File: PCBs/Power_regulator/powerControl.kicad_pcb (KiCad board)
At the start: 2 copper layers, 37.8 x 50 mm, 33 parts, among them J1 Conn_01x03_Female, J10 Conn_01x06_Male, J11 Conn_01x04_Male, J2 Conn_01x06_Female, J3 Conn_01x04_Male, J4 Conn_01x01_Male, J5 Conn_01x01_Male, J6 Conn_01x01_Male, J7 Conn_01x01_Male, J8 Conn_01x03_Female, J9 Conn_01x04_Female, Q1 PMOS, Q2 NMOS, Q3 Q_NMOS_GSD, Q4 Q_PMOS_GSD, Q5 Q_NMOS_GSD, U1 MAX9938

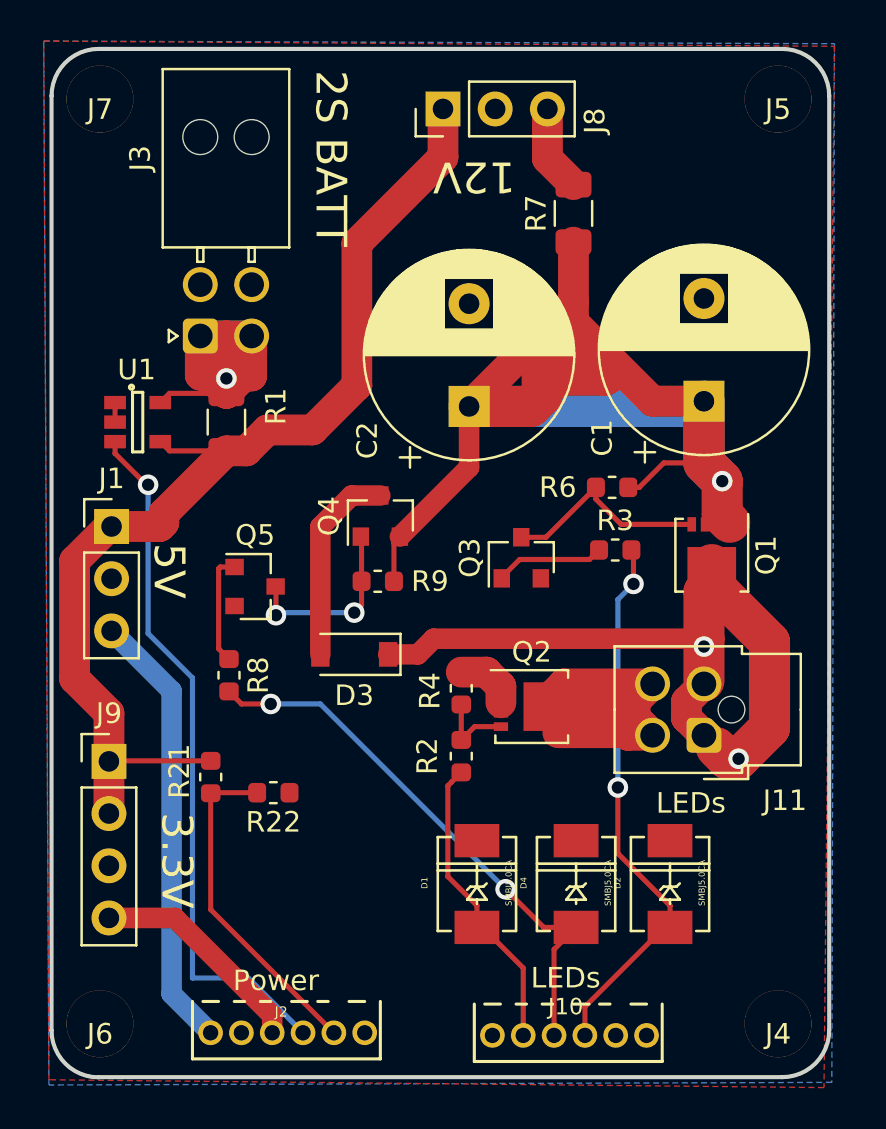
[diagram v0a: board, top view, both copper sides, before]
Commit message: Update for revision05a
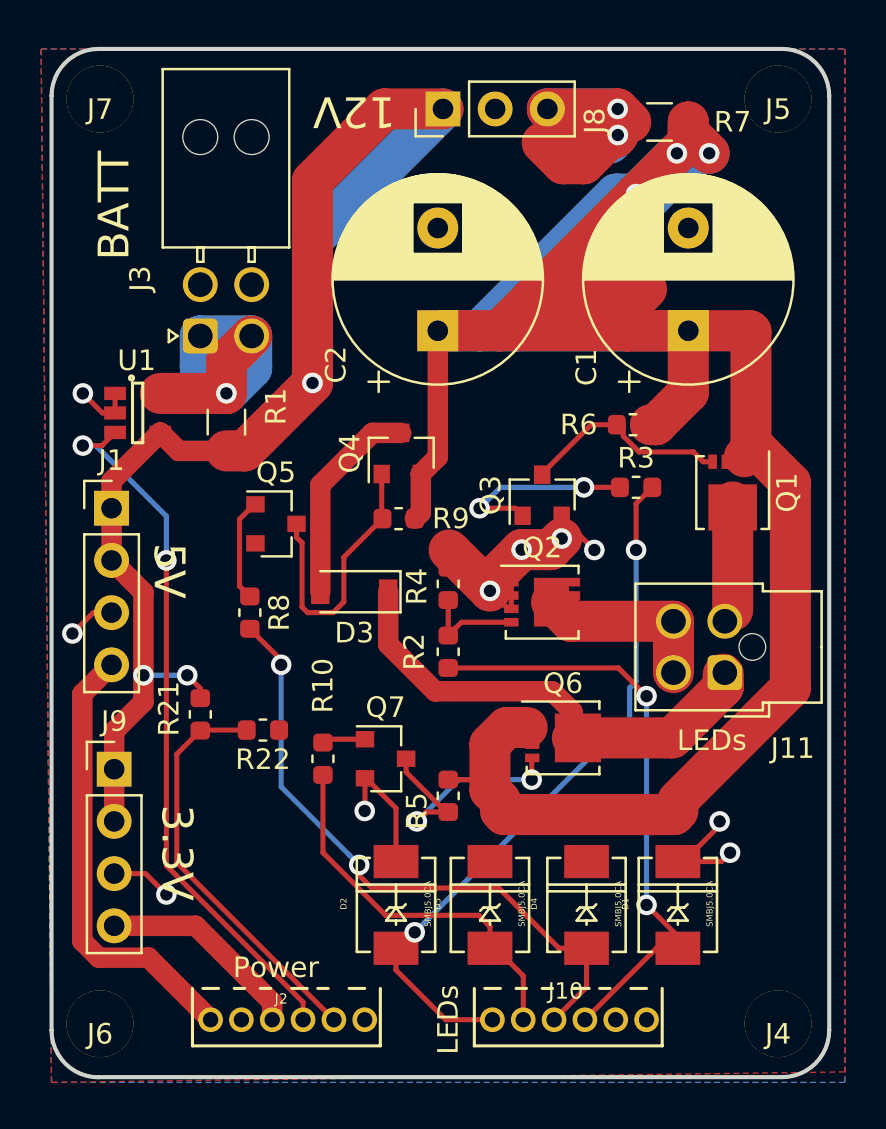
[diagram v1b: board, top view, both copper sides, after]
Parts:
- added D5: SMBJ5.0CA, myLib:DO-214AA, F.Cu at (94.0, 77.2)
- added Q6: PMOS, Package_SON:Diodes_PowerDI3333-8, F.Cu at (97.5, 69.1)
- added Q7: Q_NMOS_GSD, Package_TO_SOT_SMD:SOT-23, F.Cu at (88.9, 70.1)
- added R10: 400R, Resistor_SMD:R_0603_1608Metric, F.Cu at (85.9, 70.1)
- added R5: 10k, Resistor_SMD:R_0603_1608Metric, F.Cu at (91.9, 71.9)
- J1: value Conn_01x03_Female -> Conn_01x04_Female; footprint Connector_PinHeader_2.54mm:PinHeader_1x03_P2.54mm_Vertical -> Connector_PinHeader_2.54mm:PinHeader_1x04_P2.54mm_Vertical
- moved D2 13.4 mm to (89.4, 77.2)
- moved D1 9.83 mm to (103.1, 77.2)
- moved R7 6.11 mm to (102.2, 39.1), turned to 180 degrees
- moved R2 5.12 mm to (91.9, 64.9)
- moved R4 5.12 mm to (91.9, 61.6)
- moved Q2 5.11 mm to (96.5, 62.5)
- moved C2 3.99 mm to (91.4, 49.3)
- moved C1 3.51 mm to (103.6, 49.3)
- moved R8 3.21 mm to (82.3, 63.0)
- moved Q4 3.21 mm to (89.7, 55.2)
- moved Q5 3.21 mm to (83.6, 58.7)
- moved R3 3.21 mm to (101.1, 56.9)
- moved J11 3.21 mm to (105.4, 65.9)
- moved Q1 3.21 mm to (105.8, 57.1)
- moved Q3 3.21 mm to (96.5, 57.3)
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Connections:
- D1 pad 1: LED_EN -> Flash
- D2 pad 1: Flash -> LED_EN2
- D3 pad 1: LED+ -> LED1+
- J1 pad 2: GND -> /Vbatt_out
- J1 pad 3: /5V -> GND
- J10 pad 5: LED_EN -> LED_EN1
- J10 pad 6: LED_Sense -> LED_EN2
- J11 pad 1: LED+ -> LED1+
- J11 pad 2: LED+ -> LED2+
- Q1 pad 5: LED+ -> LED2+
- R2 pad 2: LED_EN -> Flash
- R3 pad 2: Flash -> LED_EN2
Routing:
- net V_LED: track 65.9 -> 140.1 mm, vias 1 -> 3
- net LED+: track 40.3 -> 0.00 mm, vias 2 -> 0
- net LED_EN2: track 0.00 -> 34.4 mm, vias 0 -> 2
- net GND: track 3.96 -> 35.7 mm, vias 0 -> 10
- net LED1+: track 0.00 -> 23.2 mm
- net LED_EN1: track 0.00 -> 18.8 mm
- net /12V: track 4.21 -> 20.7 mm, vias 0 -> 2
- net LED_EN: track 14.8 -> 0.00 mm
- net /Vbatt_out: track 54.1 -> 67.4 mm, vias 0 -> 3
- net Net-(Q6-Pad4): track 0.00 -> 12.7 mm, vias 0 -> 2
- net LED-: track 19.8 -> 8.82 mm
- net /Vbatt_in: track 23.4 -> 15.6 mm
- net LED2+: track 0.00 -> 5.28 mm
- net Net-(Q4-Pad1): track 9.13 -> 13.5 mm, vias 2 -> 0
- net Net-(Q3-Pad1): track 5.34 -> 9.50 mm, vias 0 -> 2
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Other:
- board text added: "BATT"
- board text added: "March 2020"
- board text added: "Power Controller rev04a"
- board text removed: "2S BATT"
- board text removed: "June 25, 2019"
- board text removed: "Power Controller rev03a"

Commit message: Update for BES publication
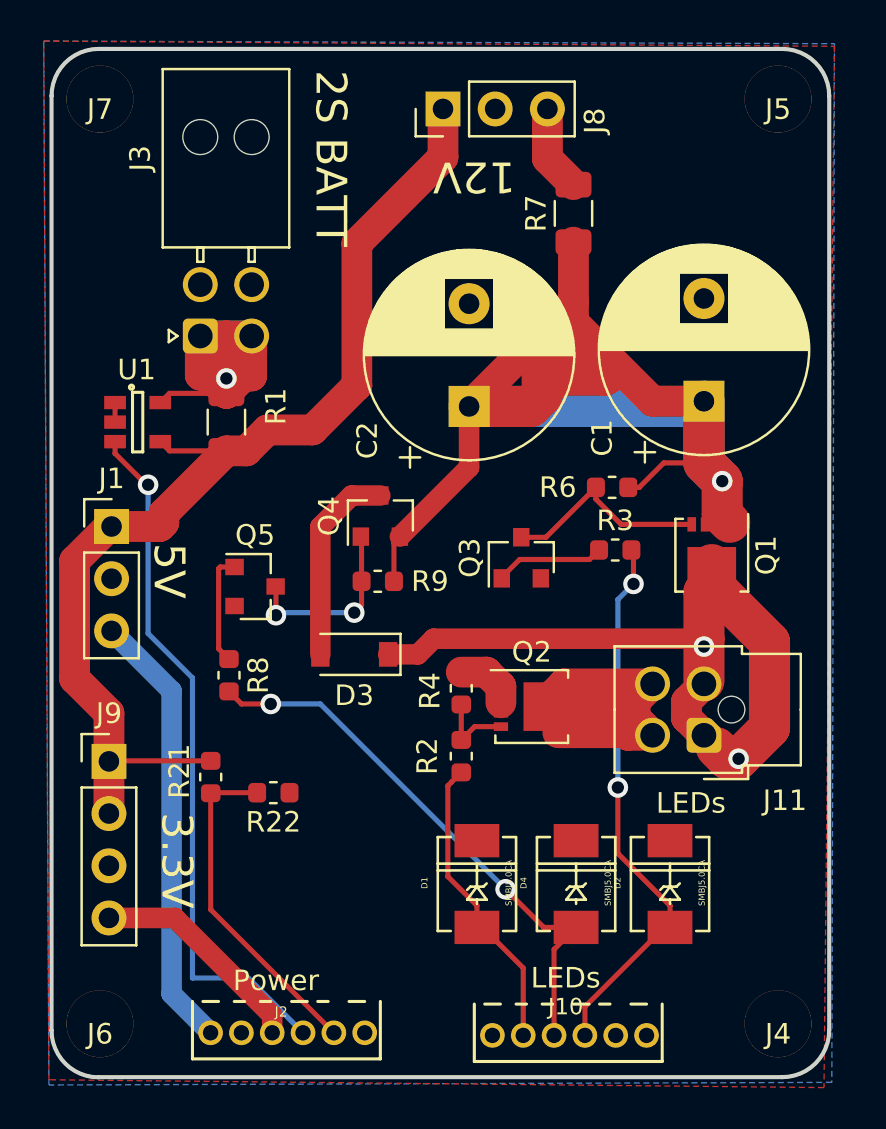
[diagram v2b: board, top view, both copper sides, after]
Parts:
- removed D5: SMBJ5.0CA, myLib:DO-214AA
- removed Q6: PMOS, Package_SON:Diodes_PowerDI3333-8
- removed Q7: Q_NMOS_GSD, Package_TO_SOT_SMD:SOT-23
- removed R10: 400R, Resistor_SMD:R_0603_1608Metric
- removed R5: 10k, Resistor_SMD:R_0603_1608Metric
- J1: value Conn_01x04_Female -> Conn_01x03_Female; footprint Connector_PinHeader_2.54mm:PinHeader_1x04_P2.54mm_Vertical -> Connector_PinHeader_2.54mm:PinHeader_1x03_P2.54mm_Vertical
- moved D2 13.4 mm to (102.7, 76.2)
- moved D1 9.83 mm to (93.3, 76.2)
- moved R7 6.11 mm to (98.0, 43.6), turned to 90 degrees
- moved R2 5.12 mm to (92.6, 70.0)
- moved R4 5.12 mm to (92.6, 66.7)
- moved Q2 5.11 mm to (96.0, 67.6)
- moved C2 3.99 mm to (93.0, 53.0)
- moved C1 3.51 mm to (104.4, 52.7)
- moved R8 3.21 mm to (81.3, 66.0)
- moved Q4 3.21 mm to (88.6, 58.3)
- moved Q5 3.21 mm to (82.5, 61.7)
- moved R3 3.21 mm to (100.1, 59.9)
- moved J11 3.21 mm to (104.4, 69.0)
- moved Q1 3.21 mm to (104.8, 60.2)
- moved Q3 3.21 mm to (95.5, 60.3)
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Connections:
- D1 pad 1: Flash -> LED_EN
- D2 pad 1: LED_EN2 -> Flash
- D3 pad 1: LED1+ -> LED+
- J1 pad 2: /Vbatt_out -> GND
- J1 pad 3: GND -> /5V
- J10 pad 5: LED_EN1 -> LED_EN
- J10 pad 6: LED_EN2 -> LED_Sense
- J11 pad 1: LED1+ -> LED+
- J11 pad 2: LED2+ -> LED+
- Q1 pad 5: LED2+ -> LED+
- R2 pad 2: Flash -> LED_EN
- R3 pad 2: LED_EN2 -> Flash
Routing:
- net V_LED: track 140.1 -> 65.9 mm, vias 3 -> 1
- net LED+: track 0.00 -> 40.3 mm, vias 0 -> 2
- net LED_EN2: track 34.4 -> 0.00 mm, vias 2 -> 0
- net GND: track 35.7 -> 3.96 mm, vias 10 -> 0
- net LED1+: track 23.2 -> 0.00 mm
- net LED_EN1: track 18.8 -> 0.00 mm
- net /12V: track 20.7 -> 4.21 mm, vias 2 -> 0
- net LED_EN: track 0.00 -> 14.8 mm
- net /Vbatt_out: track 67.4 -> 54.1 mm, vias 3 -> 0
- net Net-(Q6-Pad4): track 12.7 -> 0.00 mm, vias 2 -> 0
- net LED-: track 8.82 -> 19.8 mm
- net /Vbatt_in: track 15.6 -> 23.4 mm
- net LED2+: track 5.28 -> 0.00 mm
- net Net-(Q4-Pad1): track 13.5 -> 9.13 mm, vias 0 -> 2
- net Net-(Q3-Pad1): track 9.50 -> 5.34 mm, vias 2 -> 0
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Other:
- board text added: "2S BATT"
- board text added: "June 25, 2019"
- board text added: "Power Controller rev03a"
- board text removed: "BATT"
- board text removed: "March 2020"
- board text removed: "Power Controller rev04a"
